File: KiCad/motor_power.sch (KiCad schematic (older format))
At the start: 29 parts, among them U1 DPS1133FIA-13, U4 TBD62783A

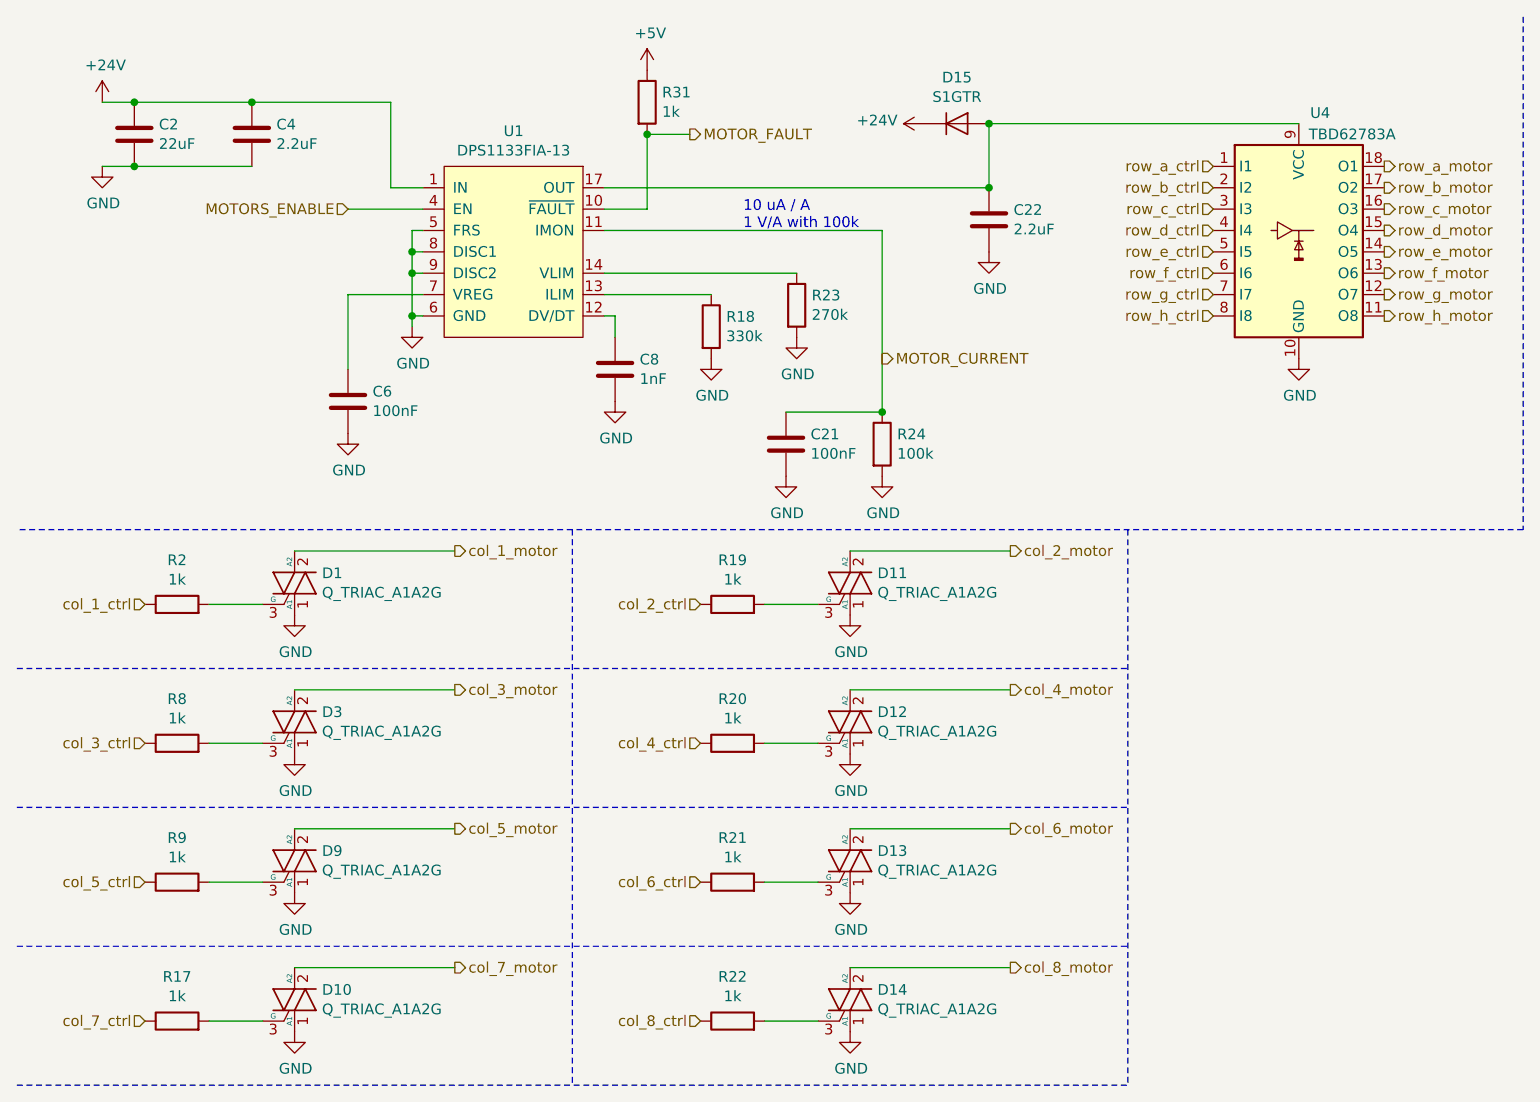
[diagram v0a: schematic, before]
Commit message: Making some board modifications for the final revision
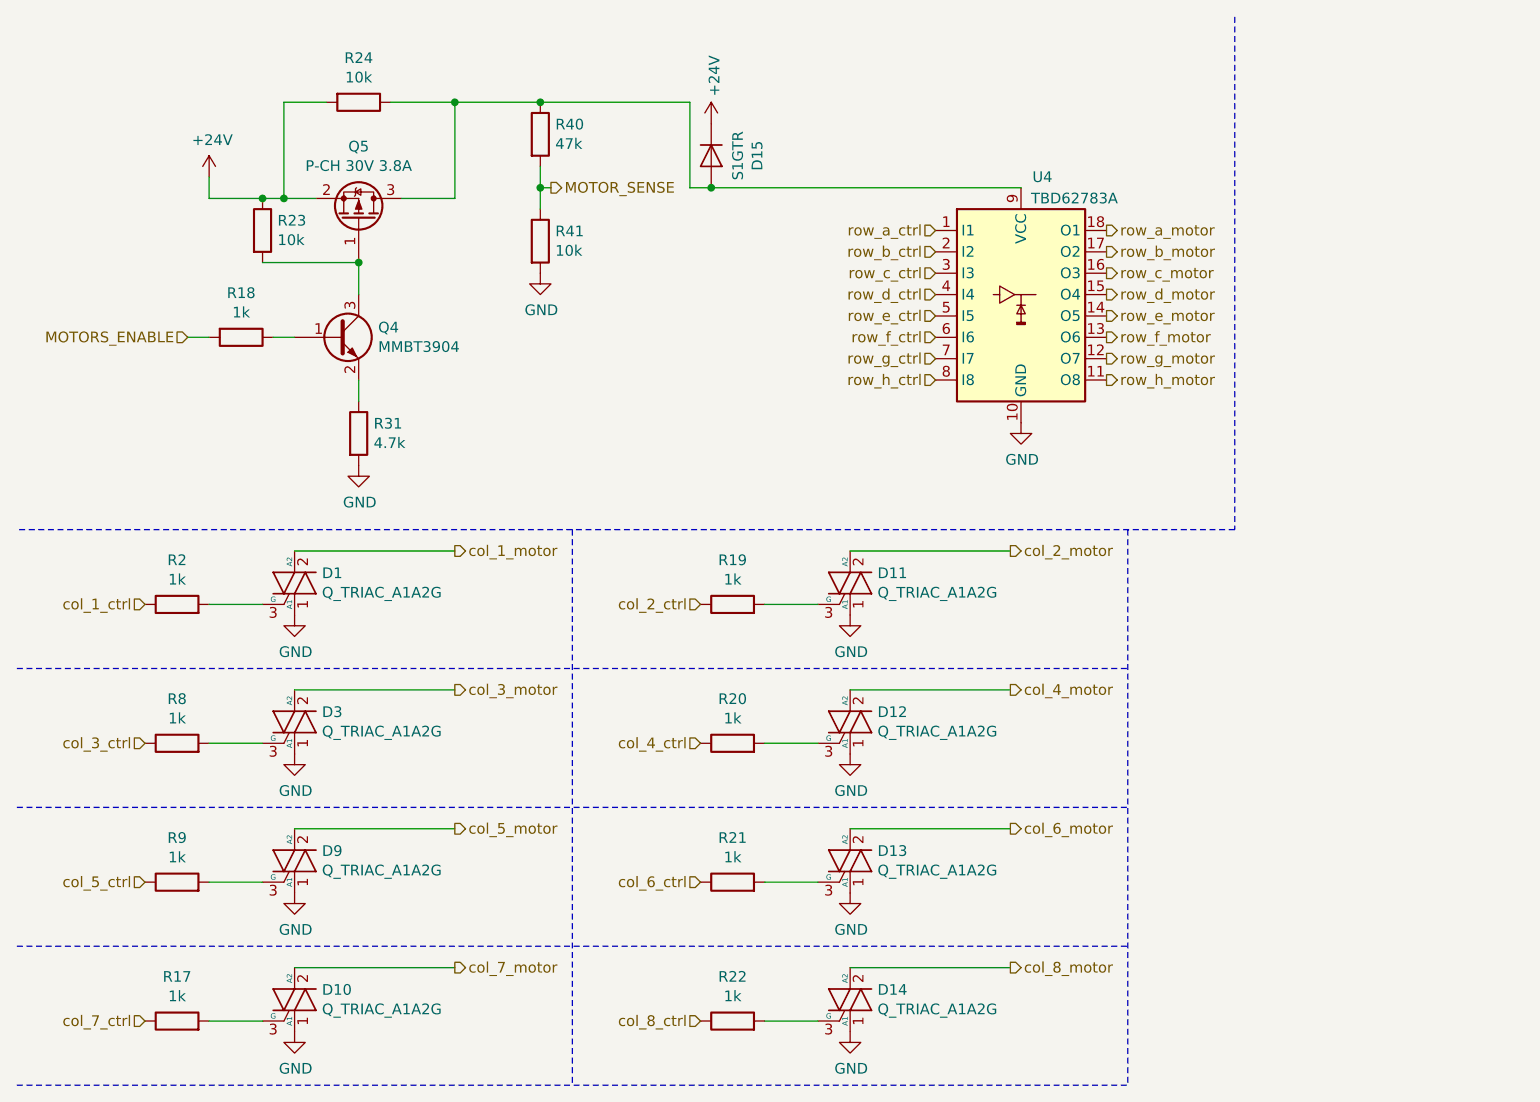
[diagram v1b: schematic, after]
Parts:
- removed C2: 22uF, Capacitor_SMD:C_1210_3225Metric_Pad1.42x2.65mm_HandSolder, symbol Device:C
- removed C21, C6: 100nF, Capacitor_SMD:C_0603_1608Metric_Pad1.05x0.95mm_HandSolder, symbol Device:C
- removed C22, C4: 2.2uF, Capacitor_SMD:C_0603_1608Metric_Pad1.05x0.95mm_HandSolder, symbol Device:C
- removed C8: 1nF, Capacitor_SMD:C_0603_1608Metric_Pad1.05x0.95mm_HandSolder, symbol Device:C
- removed U1: DPS1133FIA-13, Snack Machine:DPS1133FIA-13, symbol Snack_Machine:DPS1133FIA-13
- added Q4: MMBT3904, Snack Machine:SOT-23_Handsoldering_Lite, symbol Transistor_BJT:MMBT3904
- added Q5: P-CH 30V 3.8A, Snack Machine:SOT-23_Handsoldering_Lite, symbol Device:Q_PMOS_GSD
- added R40: 47k, Resistor_SMD:R_0603_1608Metric_Pad1.05x0.95mm_HandSolder, symbol Device:R
- added R41: 10k, Resistor_SMD:R_0603_1608Metric_Pad1.05x0.95mm_HandSolder, symbol Device:R
- R18: value 330k -> 1k; Bin 20 -> (none); Manufacturer Yageo -> (none); Part Number RC0603FR-07330KL -> (none)
- R23: value 270k -> 10k; Bin 21 -> (none); Manufacturer Yageo -> (none); Part Number RC0603FR-07270KL -> (none)
- R24: value 100k -> 10k; Bin 16 -> (none); Manufacturer Yageo -> (none); Part Number RC0603FR-07100KL -> (none)
- R31: value 1k -> 4.7k; Bin 1 -> (none); Manufacturer Yageo -> (none); Part Number RC0603FR-071KL -> (none)
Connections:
- net MOTOR_CURRENT is gone; now on an unnamed net: R24.1
- net MOTOR_FAULT is gone; now on net GND: R31.2
- net +24V: now also R23.1, R24.2, Q5.2 (S)
- net GND: now also R41.2; no longer R18.2, R23.2, R24.2
- net MOTORS_ENABLE: now also R18.2
- net at D15.2 (A), U4.9 (VCC): now also Q5.3 (D), R40.1
- net at R18.1: now also Q4.1 (B)
- net +5V: no longer names the net of R31.1
- net +5V: now also Q4.2 (E)
- new net: Q4.3 (C), Q5.1 (G), R23.2
- new net MOTOR_SENSE: R40.2, R41.1
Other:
- note removed: "10 uA / A\n1 V/A with 100k"
- moved on the sheet: D15, U4

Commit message: Committing changes to the circuit board
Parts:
- R18: Bin (none) -> 1; Manufacturer (none) -> Yageo; Part Number (none) -> RC0603FR-071KL
- R23, R24, R41: Bin (none) -> 10; Manufacturer (none) -> Yageo; Part Number (none) -> RC0603FR-0710KL
- R31: Bin (none) -> 5; Manufacturer (none) -> Yageo; Part Number (none) -> RC0603FR-074K7L
- R40: Bin (none) -> 36; Manufacturer (none) -> Yageo; Part Number (none) -> RC0603FR-0747KL
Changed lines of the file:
@@
 F 2 "Resistor_SMD:R_0603_1608Metric_Pad1.05x0.95mm_HandSolder" V 1430 1950 50  0001 C CNN
 F 3 "~" H 1500 1950 50  0001 C CNN
+F 4 "Yageo" V 1500 1950 50  0001 C CNN "Manufacturer"
+F 5 "RC0603FR-071KL" V 1500 1950 50  0001 C CNN "Part Number"
+F 6 "1" V 1500 1950 50  0001 C CNN "Bin"
 	1    1500 1950
 	0    1    1    0
@@
 F 2 "Resistor_SMD:R_0603_1608Metric_Pad1.05x0.95mm_HandSolder" V 1980 2400 50  0001 C CNN
 F 3 "~" H 2050 2400 50  0001 C CNN
+F 4 "Yageo" H 2050 2400 50  0001 C CNN "Manufacturer"
+F 5 "RC0603FR-074K7L" H 2050 2400 50  0001 C CNN "Part Number"
+F 6 "5" H 2050 2400 50  0001 C CNN "Bin"
 	1    2050 2400
 	1    0    0    -1
@@
 F 2 "Resistor_SMD:R_0603_1608Metric_Pad1.05x0.95mm_HandSolder" V 1530 1450 50  0001 C CNN
 F 3 "~" H 1600 1450 50  0001 C CNN
+F 4 "RC0603FR-0710KL" H 1600 1450 50  0001 C CNN "Part Number"
+F 5 "Yageo" H 1600 1450 50  0001 C CNN "Manufacturer"
+F 6 "10" H 1600 1450 50  0001 C CNN "Bin"
 	1    1600 1450
 	1    0    0    -1
@@
 F 2 "Resistor_SMD:R_0603_1608Metric_Pad1.05x0.95mm_HandSolder" V 1980 850 50  0001 C CNN
 F 3 "~" H 2050 850 50  0001 C CNN
+F 4 "Yageo" V 2050 850 50  0001 C CNN "Manufacturer"
+F 5 "RC0603FR-0710KL" V 2050 850 50  0001 C CNN "Part Number"
+F 6 "10" V 2050 850 50  0001 C CNN "Bin"
 	1    2050 850
 	0    1    1    0
@@
 F 2 "Resistor_SMD:R_0603_1608Metric_Pad1.05x0.95mm_HandSolder" V 2830 1000 50  0001 C CNN
 F 3 "~" H 2900 1000 50  0001 C CNN
+F 4 "36" H 2900 1000 50  0001 C CNN "Bin"
+F 5 "Yageo" H 2900 1000 50  0001 C CNN "Manufacturer"
+F 6 "RC0603FR-0747KL" H 2900 1000 50  0001 C CNN "Part Number"
 	1    2900 1000
 	1    0    0    -1
@@
 F 2 "Resistor_SMD:R_0603_1608Metric_Pad1.05x0.95mm_HandSolder" V 2830 1500 50  0001 C CNN
 F 3 "~" H 2900 1500 50  0001 C CNN
+F 4 "RC0603FR-0710KL" H 2900 1500 50  0001 C CNN "Part Number"
+F 5 "Yageo" H 2900 1500 50  0001 C CNN "Manufacturer"
+F 6 "10" H 2900 1500 50  0001 C CNN "Bin"
 	1    2900 1500
 	1    0    0    -1
